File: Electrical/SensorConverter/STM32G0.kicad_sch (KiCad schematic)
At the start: 15 parts, among them U3 24CS256T-I/OT, U7 STM32G0B1CEUx

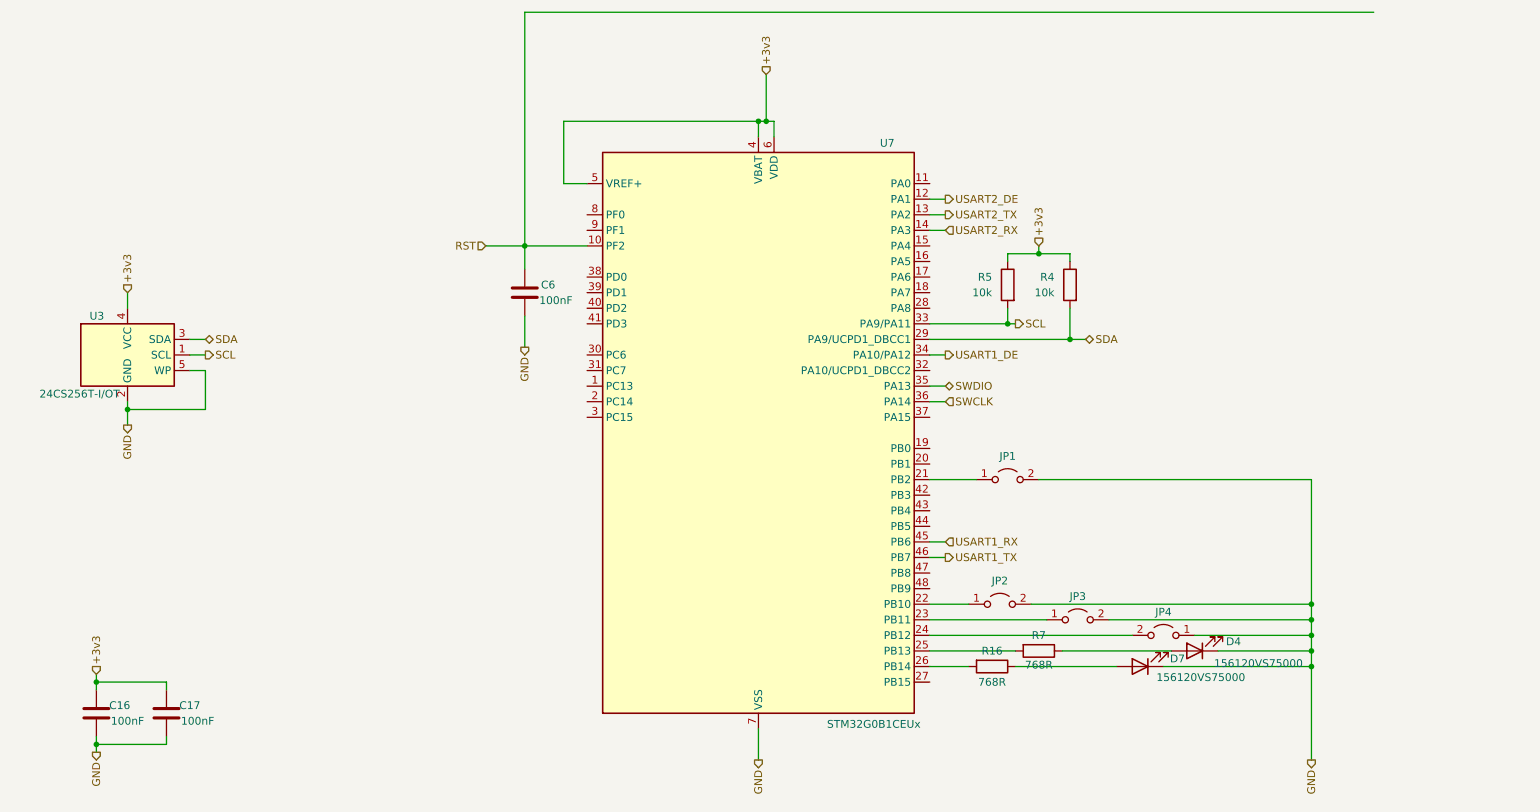
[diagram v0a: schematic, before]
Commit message: WIP
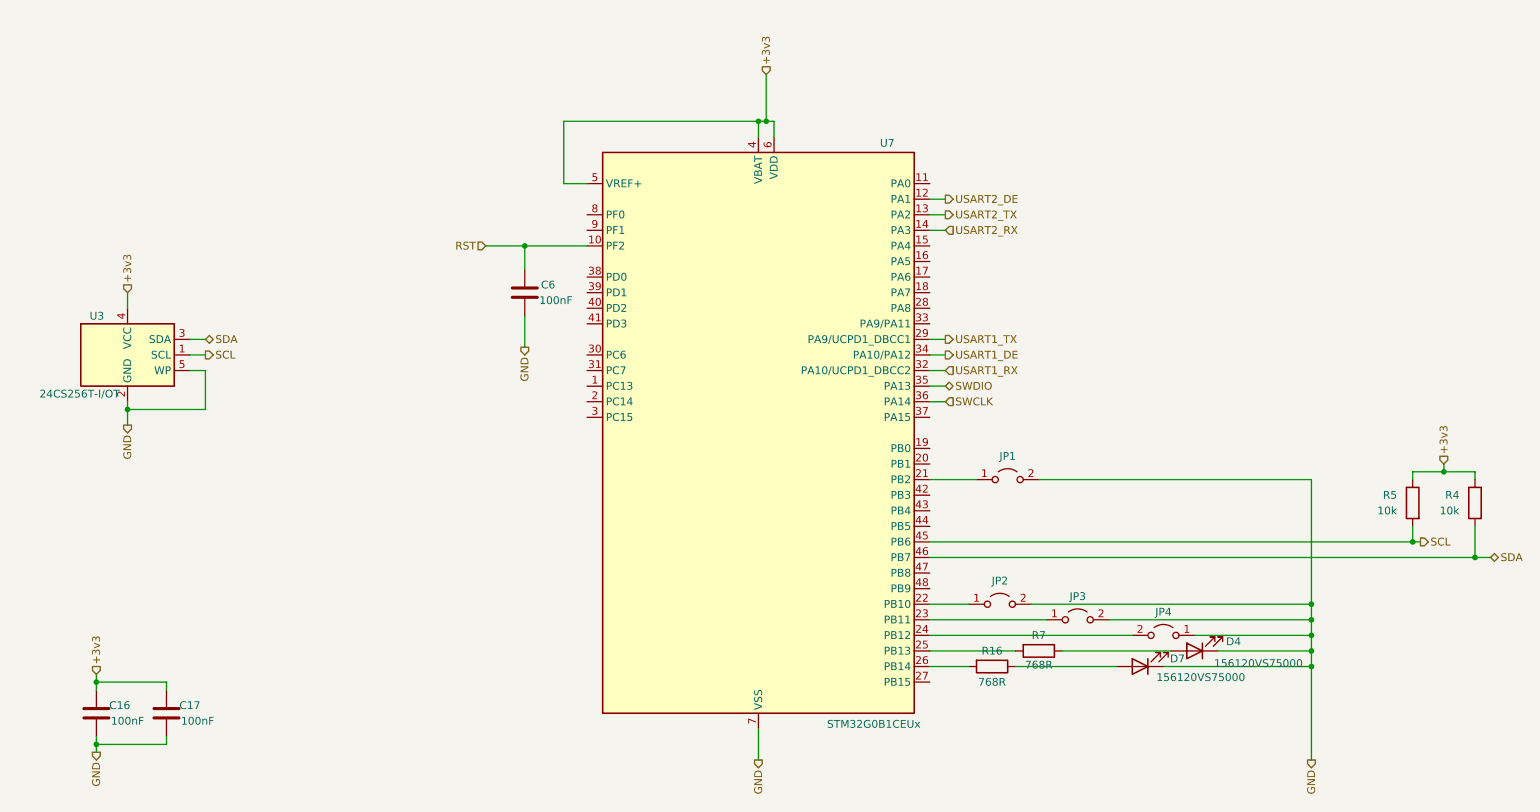
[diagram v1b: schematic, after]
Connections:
- net SCL: now also U7.45 (PB6); no longer U7.33 (PA9/PA11)
- net SDA: now also U7.46 (PB7); no longer U7.29 (PA9/UCPD1_DBCC1)
- net USART1_RX: now also U7.32 (PA10/UCPD1_DBCC2); no longer U7.45 (PB6)
- net USART1_TX: now also U7.29 (PA9/UCPD1_DBCC1); no longer U7.46 (PB7)
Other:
- moved on the sheet: R4, R5
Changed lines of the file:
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@@
 	(paper "A4")
 	(junction
-		(at 200.66 73.66)
+		(at 266.7 109.22)
 		(diameter 0)
 		(color 0 0 0 0)
@@
 	)
 	(junction
-		(at 190.5 71.12)
+		(at 256.54 106.68)
 		(diameter 0)
 		(color 0 0 0 0)
@@
 	)
 	(junction
-		(at 195.58 59.69)
+		(at 261.62 95.25)
 		(diameter 0)
 		(color 0 0 0 0)
@@
 	(wire
 		(pts
-			(xy 177.8 109.22) (xy 180.34 109.22)
-		)
-		(stroke
-			(width 0)
-			(type default)
-		)
-	)
-	(wire
-		(pts
-			(xy 200.66 73.66) (xy 200.66 68.58)
+			(xy 177.8 109.22) (xy 266.7 109.22)
+		)
+		(stroke
+			(width 0)
+			(type default)
+		)
+	)
+	(wire
+		(pts
+			(xy 177.8 73.66) (xy 180.34 73.66)
+		)
+		(stroke
+			(width 0)
+			(type default)
+		)
+	)
+	(wire
+		(pts
+			(xy 266.7 109.22) (xy 266.7 104.14)
 		)
 		(stroke
@@
 	(wire
 		(pts
-			(xy 195.58 58.42) (xy 195.58 59.69)
+			(xy 261.62 93.98) (xy 261.62 95.25)
 		)
 		(stroke
@@
 	(wire
 		(pts
-			(xy 190.5 71.12) (xy 191.77 71.12)
+			(xy 256.54 106.68) (xy 257.81 106.68)
 		)
 		(stroke
@@
 	(wire
 		(pts
-			(xy 200.66 60.96) (xy 200.66 59.69)
+			(xy 266.7 96.52) (xy 266.7 95.25)
 		)
 		(stroke
@@
 	(wire
 		(pts
-			(xy 200.66 73.66) (xy 203.2 73.66)
+			(xy 266.7 109.22) (xy 269.24 109.22)
 		)
 		(stroke
@@
 	(wire
 		(pts
-			(xy 177.8 73.66) (xy 200.66 73.66)
-		)
-		(stroke
-			(width 0)
-			(type default)
-		)
-	)
-	(wire
-		(pts
 			(xy 240.03 127) (xy 240.03 142.24)
 		)
@@
 	(wire
 		(pts
-			(xy 200.66 59.69) (xy 195.58 59.69)
+			(xy 266.7 95.25) (xy 261.62 95.25)
 		)
 		(stroke
@@
 	(wire
 		(pts
-			(xy 111.76 20.32) (xy 111.76 58.42)
-		)
-		(stroke
-			(width 0)
-			(type default)
-		)
-	)
-	(wire
-		(pts
-			(xy 250.19 20.32) (xy 111.76 20.32)
-		)
-		(stroke
-			(width 0)
-			(type default)
-		)
-	)
-	(wire
-		(pts
 			(xy 215.9 127) (xy 240.03 127)
 		)
@@
 	(wire
 		(pts
-			(xy 177.8 106.68) (xy 180.34 106.68)
-		)
-		(stroke
-			(width 0)
-			(type default)
-		)
-	)
-	(wire
-		(pts
-			(xy 190.5 60.96) (xy 190.5 59.69)
+			(xy 177.8 78.74) (xy 180.34 78.74)
+		)
+		(stroke
+			(width 0)
+			(type default)
+		)
+	)
+	(wire
+		(pts
+			(xy 177.8 106.68) (xy 256.54 106.68)
+		)
+		(stroke
+			(width 0)
+			(type default)
+		)
+	)
+	(wire
+		(pts
+			(xy 256.54 96.52) (xy 256.54 95.25)
 		)
 		(stroke
@@
 	(wire
 		(pts
-			(xy 195.58 59.69) (xy 190.5 59.69)
+			(xy 261.62 95.25) (xy 256.54 95.25)
 		)
 		(stroke
@@
 	(wire
 		(pts
-			(xy 177.8 71.12) (xy 190.5 71.12)
-		)
-		(stroke
-			(width 0)
-			(type default)
-		)
-	)
-	(wire
-		(pts
 			(xy 177.8 83.82) (xy 180.34 83.82)
 		)
@@
 	(wire
 		(pts
-			(xy 190.5 68.58) (xy 190.5 71.12)
+			(xy 256.54 104.14) (xy 256.54 106.68)
 		)
 		(stroke
@@
 	(hierarchical_label "SCL"
 		(shape output)
-		(at 191.77 71.12 0)
+		(at 257.81 106.68 0)
 		(effects
 			(font
@@
 	(hierarchical_label "SDA"
 		(shape bidirectional)
-		(at 203.2 73.66 0)
+		(at 269.24 109.22 0)
 		(effects
 			(font
@@
 	(hierarchical_label "USART1_TX"
 		(shape output)
-		(at 180.34 109.22 0)
+		(at 180.34 73.66 0)
 		(effects
 			(font
@@
 	(hierarchical_label "USART1_RX"
 		(shape input)
-		(at 180.34 106.68 0)
+		(at 180.34 78.74 0)
 		(effects
 			(font
@@
 	(hierarchical_label "+3v3"
 		(shape input)
-		(at 195.58 58.42 90)
+		(at 261.62 93.98 90)
 		(effects
 			(font
@@
 	(symbol
 		(lib_id "Device:R")
-		(at 200.66 64.77 0)
+		(at 266.7 100.33 0)
 		(mirror y)
 		(unit 1)
@@
 		(fields_autoplaced yes)
 		(property "Reference" "R4"
-			(at 198.12 63.4999 0)
+			(at 264.16 99.0599 0)
 			(effects
 				(font
@@
 		)
 		(property "Value" "10k"
-			(at 198.12 66.0399 0)
+			(at 264.16 101.5999 0)
 			(effects
 				(font
@@
 		)
 		(property "Footprint" "Resistor_SMD:R_0402_1005Metric"
-			(at 202.438 64.77 90)
+			(at 268.478 100.33 90)
 			(effects
 				(font
@@
 		)
 		(property "Datasheet" "~"
-			(at 200.66 64.77 0)
+			(at 266.7 100.33 0)
 			(effects
 				(font
@@
 		)
 		(property "Description" ""
-			(at 200.66 64.77 0)
+			(at 266.7 100.33 0)
 			(effects
 				(font
@@
 	(symbol
 		(lib_id "Device:R")
-		(at 190.5 64.77 0)
+		(at 256.54 100.33 0)
 		(mirror y)
 		(unit 1)
@@
 		(fields_autoplaced yes)
 		(property "Reference" "R5"
-			(at 187.96 63.4999 0)
+			(at 254 99.0599 0)
 			(effects
 				(font
@@
 		)
 		(property "Value" "10k"
-			(at 187.96 66.0399 0)
+			(at 254 101.5999 0)
 			(effects
 				(font
@@
 		)
 		(property "Footprint" "Resistor_SMD:R_0402_1005Metric"
-			(at 192.278 64.77 90)
+			(at 258.318 100.33 90)
 			(effects
 				(font
@@
 		)
 		(property "Datasheet" "~"
-			(at 190.5 64.77 0)
+			(at 256.54 100.33 0)
 			(effects
 				(font
@@
 		)
 		(property "Description" ""
-			(at 190.5 64.77 0)
-			(effects
-				(font
+			(at 256.54 100.33 0)
+			(effects
+				(font
